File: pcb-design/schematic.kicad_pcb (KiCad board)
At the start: 2 copper layers, 73 parts, among them J4 Screw_Terminal_01x02, J6 Conn_02x13_Top_Bottom, Q1 2N2222, Q2 2N2222, Q3 2N2222, Q6 2N2222, Q8 2N3906, U2 MCP23017_SP, U3 MCP2562-E-P, U4 AP1117-33, U6 ESP32-DEVKITC-32D

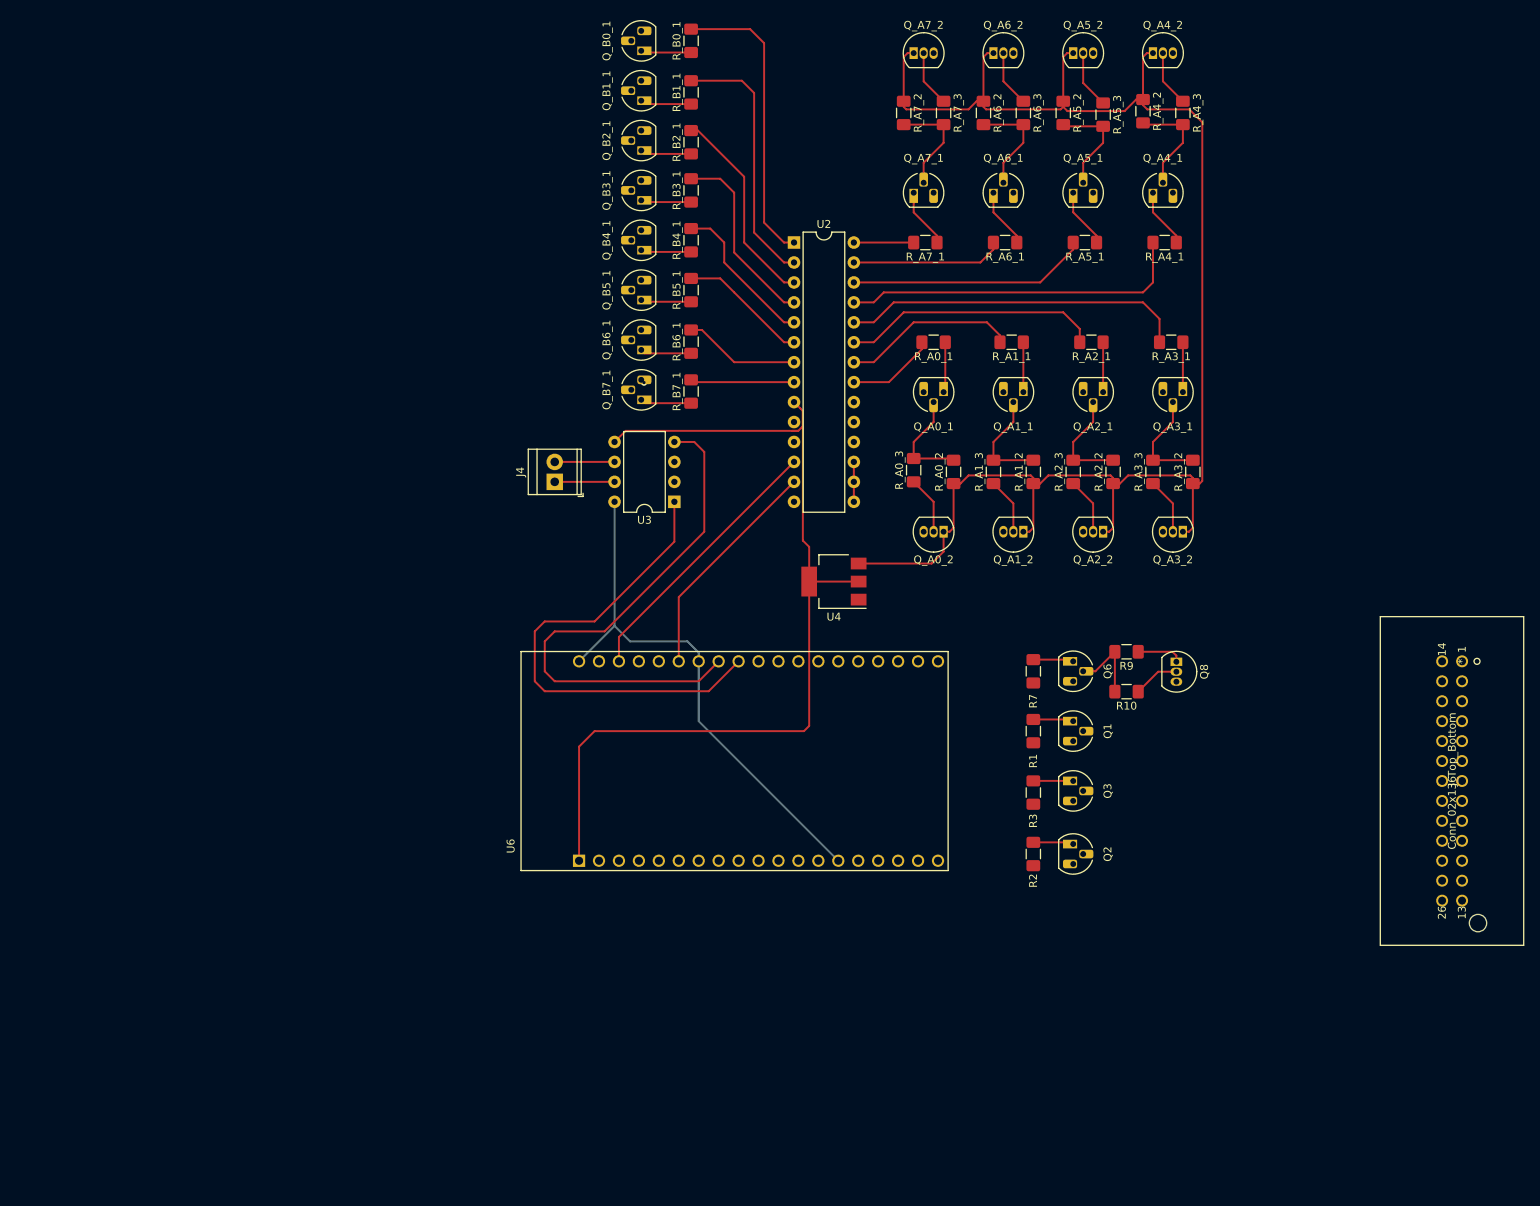
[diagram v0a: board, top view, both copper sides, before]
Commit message: Final changes for Rev 1 board, ordered 10/06/2020
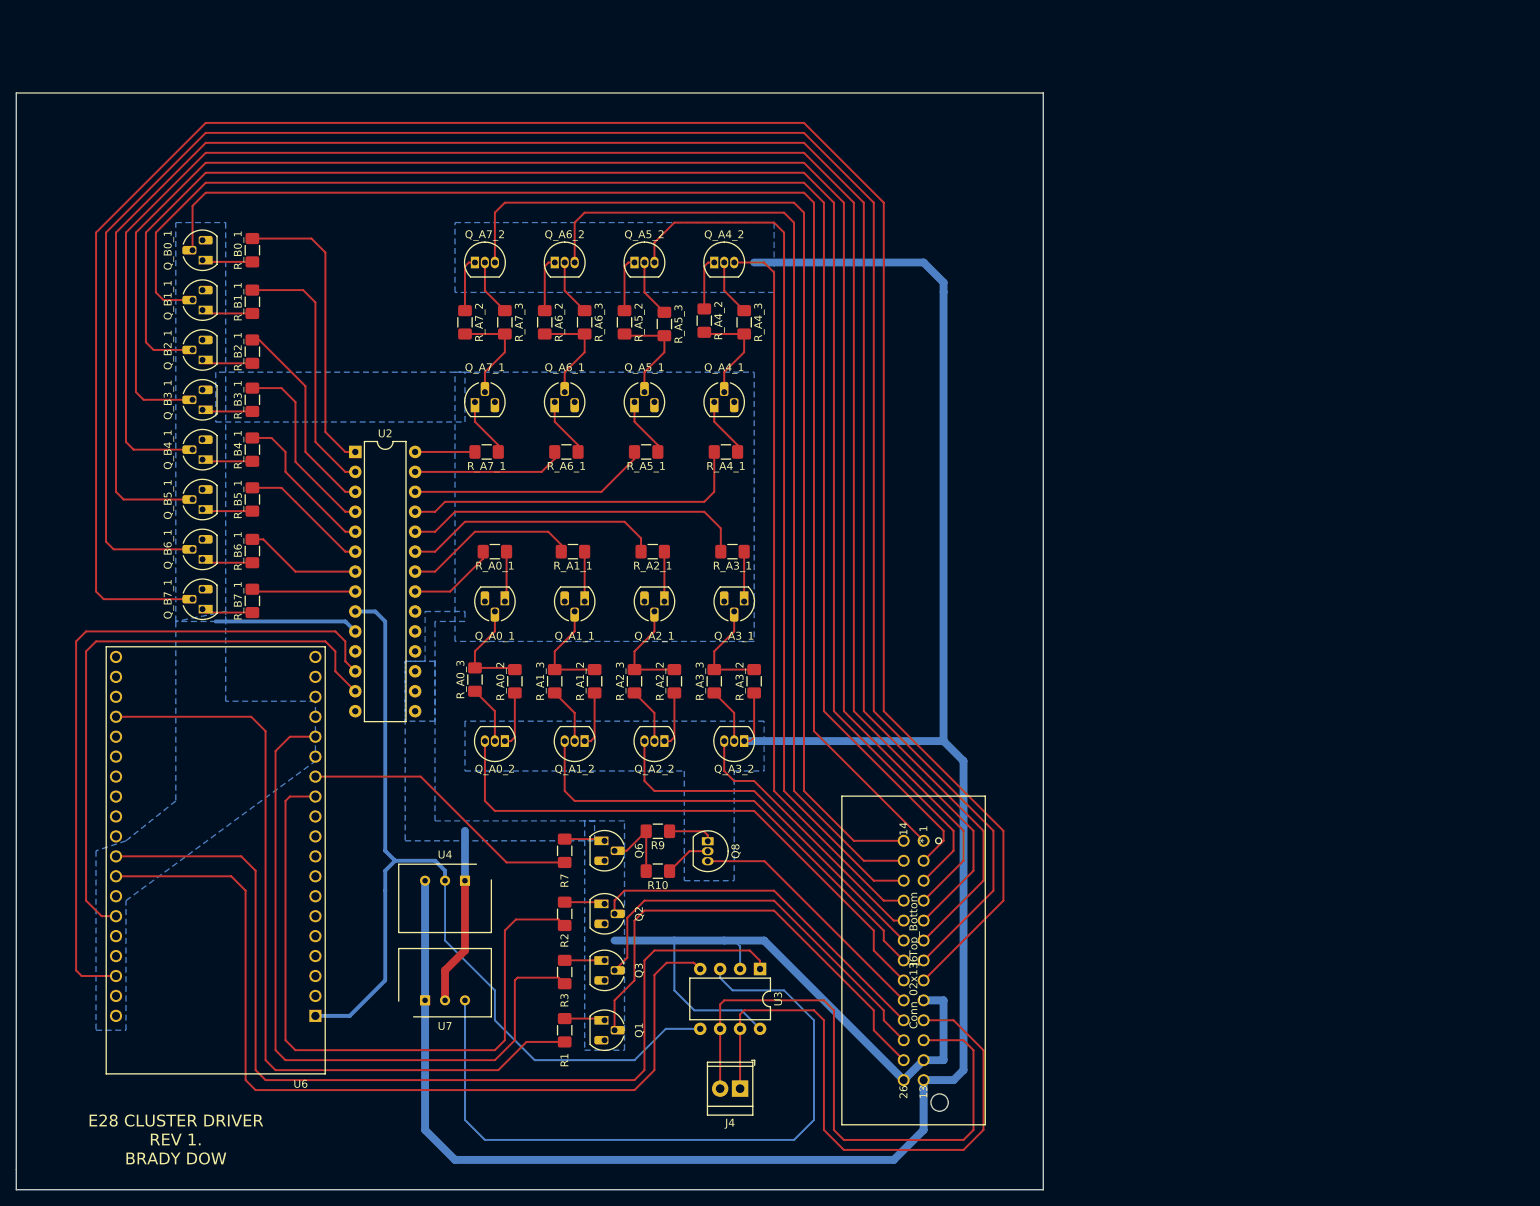
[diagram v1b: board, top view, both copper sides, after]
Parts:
- added U7: L7805, Package_SIP:SIP3_11.6x8.5mm, F.Cu at (96.5, 147.3)
- U4: footprint Package_TO_SOT_SMD:SOT-223-3_TabPin2 -> Package_SIP:SIP3_11.6x8.5mm
- moved J4 80.8 mm to (136.6, 158.6), turned to 180 degrees
- moved J6 72.3 mm to (160.0, 127.0)
- moved Q1 70.8 mm to (119.4, 149.9)
- moved R1 70.8 mm to (114.3, 151.1)
- moved U6 67.3 mm to (69.8, 129.5), turned to 180 degrees
- moved R10 63.9 mm to (126.2, 130.9)
- moved R7 63.9 mm to (114.3, 128.3)
- moved R3 63.9 mm to (114.3, 143.7)
- moved R9 63.9 mm to (126.2, 125.8)
- moved Q3 63.9 mm to (119.4, 142.2)
- moved Q6 63.9 mm to (119.4, 127.0)
- moved Q8 63.9 mm to (132.5, 127.1)
- moved R_B4_1 61.9 mm to (74.5, 77.2)
- moved R_A0_2 61.9 mm to (108.0, 106.7)
- moved R_A1_2 61.9 mm to (118.1, 106.7)
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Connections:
- J6 pad 1: A0_SourceOutput -> B0_SinkOutput
- J6 pad 14: B0_SinkOutput -> A7_SourceOutput
- J6 pad 15: B1_SinkOutput -> A6_SourceOutput
- J6 pad 16: B2_SinkOutput -> A5_SourceOutput
- J6 pad 17: B3_SinkOutput -> A4_SourceOutput
- J6 pad 18: B4_SinkOutput -> A3_SourceOutput
- J6 pad 19: B5_SinkOutput -> A2_SourceOutput
- J6 pad 2: A1_SourceOutput -> B1_SinkOutput
- J6 pad 20: B6_SinkOutput -> A1_SourceOutput
- J6 pad 21: B7_SinkOutput -> A0_SourceOutput
- J6 pad 22: TempGauge -> Tachometer
- J6 pad 23: Tachometer -> FuelGauge
- J6 pad 25: FuelGauge -> TempGauge
- J6 pad 3: A2_SourceOutput -> B2_SinkOutput
- J6 pad 4: A3_SourceOutput -> B3_SinkOutput
- J6 pad 5: A4_SourceOutput -> B4_SinkOutput
- J6 pad 6: A5_SourceOutput -> B5_SinkOutput
- J6 pad 7: A6_SourceOutput -> B6_SinkOutput
- J6 pad 8: A7_SourceOutput -> B7_SinkOutput
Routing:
- net B7_SinkOutput: track 0.00 -> 278.3 mm
- net B6_SinkOutput: track 0.00 -> 264.0 mm
- net B5_SinkOutput: track 0.00 -> 249.8 mm
- net B4_SinkOutput: track 0.00 -> 235.5 mm
- net B3_SinkOutput: track 0.00 -> 221.2 mm
- net B2_SinkOutput: track 0.00 -> 206.9 mm
- net B1_SinkOutput: track 0.00 -> 192.7 mm
- net B0_SinkOutput: track 0.00 -> 173.1 mm
- net A7_SourceOutput: track 0.00 -> 135.8 mm
- net A6_SourceOutput: track 0.00 -> 124.1 mm
- net +12V: track 201.3 -> 324.9 mm
- net A5_SourceOutput: track 0.00 -> 111.7 mm
- net TemperatureOutput: track 0.00 -> 101.8 mm
- net A4_SourceOutput: track 0.00 -> 93.9 mm
- net SpeedometerSignal: track 0.00 -> 90.4 mm
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- added copper zone on B.Cu, net +12V
- added copper zone on B.Cu, net GND
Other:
- board outline added: 130.8 x 139.7 mm
- board text added: "E28 CLUSTER DRIVER REV 1. BRADY DOW"
